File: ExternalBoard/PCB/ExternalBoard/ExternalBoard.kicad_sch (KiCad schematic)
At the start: 2 parts, among them U1 REF01CP

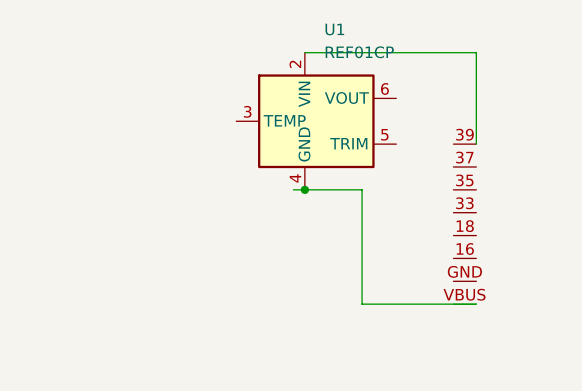
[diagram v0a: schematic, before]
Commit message: 5
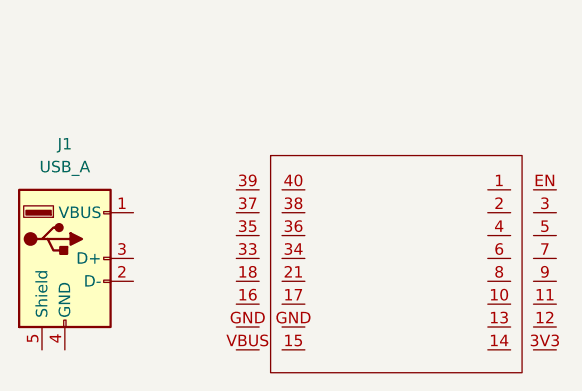
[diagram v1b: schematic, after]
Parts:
- removed U1: REF01CP, Package_DIP:DIP-8_W7.62mm, symbol Reference_Voltage:REF01CP
- added J1: USB_A, Connector_USB:USB_A_Connfly_DS1095, symbol Connector:USB_A
- D1: footprint ESP32_S2:ESP32_S2 -> (none)
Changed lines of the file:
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@@
 	(generator_version "9.0")
 	(paper "A4")
-	(junction
-		(at 96.52 99.06)
-		(diameter 0)
-		(color 0 0 0 0)
-	)
-	(wire
-		(pts
-			(xy 95.25 99.06) (xy 96.52 99.06)
+	(symbol
+		(lib_id "Connector:USB_A")
+		(at 69.85 106.68 0)
+		(unit 1)
+		(exclude_from_sim no)
+		(in_bom yes)
+		(on_board yes)
+		(dnp no)
+		(fields_autoplaced yes)
+		(property "Reference" "J1"
+			(at 69.85 93.98 0)
+			(effects
+				(font
+					(size 1.27 1.27)
+				)
+			)
 		)
-		(stroke
-			(width 0)
-			(type default)
+		(property "Value" "USB_A"
+			(at 69.85 96.52 0)
+			(effects
+				(font
+					(size 1.27 1.27)
+				)
+			)
 		)
-	)
-	(wire
-		(pts
-			(xy 102.87 99.06) (xy 102.87 111.76)
+		(property "Footprint" "Connector_USB:USB_A_Connfly_DS1095"
+			(at 73.66 107.95 0)
+			(effects
+				(font
+					(size 1.27 1.27)
+				)
+				(hide yes)
+			)
 		)
-		(stroke
-			(width 0)
-			(type default)
+		(property "Datasheet" "~"
+			(at 73.66 107.95 0)
+			(effects
+				(font
+					(size 1.27 1.27)
+				)
+				(hide yes)
+			)
 		)
-	)
-	(wire
-		(pts
-			(xy 102.87 111.76) (xy 115.57 111.76)
+		(property "Description" "USB Type A connector"
+			(at 69.85 106.68 0)
+			(effects
+				(font
+					(size 1.27 1.27)
+				)
+				(hide yes)
+			)
 		)
-		(stroke
-			(width 0)
-			(type default)
+		(pin "2"
 		)
-	)
-	(wire
-		(pts
-			(xy 96.52 99.06) (xy 102.87 99.06)
+		(pin "3"
 		)
-		(stroke
-			(width 0)
-			(type default)
+		(pin "5"
 		)
-	)
-	(wire
-		(pts
-			(xy 115.57 83.82) (xy 115.57 93.98)
+		(pin "1"
 		)
-		(stroke
-			(width 0)
-			(type default)
+		(pin "4"
 		)
-	)
-	(wire
-		(pts
-			(xy 96.52 83.82) (xy 115.57 83.82)
-		)
-		(stroke
-			(width 0)
-			(type default)
+		(instances
+			(project ""
+				(path "/1428142b-2c57-4b00-8cf4-1baa0f3d7ee6"
+					(reference "J1")
+					(unit 1)
+				)
+			)
 		)
 	)
 	(symbol
 		(lib_id "ESP32_S2:ESP32_S2")
-		(at 135.89 102.87 0)
+		(at 106.68 106.68 0)
 		(unit 1)
 		(exclude_from_sim no)
@@
 		(fields_autoplaced yes)
 		(property "Reference" "D1"
-			(at 135.89 102.87 0)
+			(at 107.95 107.95 0)
 			(effects
 				(font
@@
 		)
 		(property "Value" "~"
-			(at 113.03 91.44 0)
+			(at 106.68 92.71 0)
 			(effects
 				(font
@@
 			)
 		)
-		(property "Footprint" "ESP32_S2:ESP32_S2"
-			(at 135.89 102.87 0)
+		(property "Footprint" ""
+			(at 106.68 106.68 0)
 			(effects
 				(font
@@
 		)
 		(property "Datasheet" ""
-			(at 135.89 102.87 0)
+			(at 106.68 106.68 0)
 			(effects
 				(font
@@
 		)
 		(property "Description" ""
-			(at 135.89 102.87 0)
+			(at 106.68 106.68 0)
 			(effects
 				(font
@@
 			)
 		)
-		(pin "39"
+		(pin "21"
+		)
+		(pin "GND"
 		)
 		(pin "VBUS"
 		)
-		(pin "16"
+		(pin "4"
 		)
 		(pin "37"
 		)
-		(pin "35"
+		(pin "2"
+		)
+		(pin "39"
+		)
+		(pin "33"
+		)
+		(pin "16"
 		)
 		(pin "GND"
 		)
+		(pin "40"
+		)
 		(pin "18"
 		)
-		(pin "33"
+		(pin "38"
+		)
+		(pin "36"
+		)
+		(pin "34"
+		)
+		(pin "35"
+		)
+		(pin "17"
+		)
+		(pin "15"
+		)
+		(pin "1"
+		)
+		(pin "10"
+		)
+		(pin "9"
+		)
+		(pin "7"
+		)
+		(pin "11"
+		)
+		(pin "EN"
+		)
+		(pin "3"
+		)
+		(pin "14"
+		)
+		(pin "3V3"
+		)
+		(pin "13"
+		)
+		(pin "6"
+		)
+		(pin "12"
+		)
+		(pin "8"
+		)
+		(pin "5"
 		)
 		(instances
@@
 					(unit 1)
 				)
-			)
-		)
-	)
-	(symbol
-		(lib_id "Reference_Voltage:REF01CP")
-		(at 96.52 91.44 0)
-		(unit 1)
-		(exclude_from_sim no)
-		(in_bom yes)
-		(on_board yes)
-		(dnp no)
-		(fields_autoplaced yes)
-		(property "Reference" "U1"
-			(at 98.6633 81.28 0)
-			(effects
-				(font
-					(size 1.27 1.27)
-				)
-				(justify left)
-			)
-		)
-		(property "Value" "REF01CP"
-			(at 98.6633 83.82 0)
-			(effects
-				(font
-					(size 1.27 1.27)
-				)
-				(justify left)
-			)
-		)
-		(property "Footprint" "Package_DIP:DIP-8_W7.62mm"
-			(at 111.76 97.79 0)
-			(effects
-				(font
-					(size 1.27 1.27)
-					(italic yes)
-				)
-				(hide yes)
-			)
-		)
-		(property "Datasheet" "https://www.analog.com/media/en/technical-documentation/data-sheets/REF01_02_03.pdf"
-			(at 97.79 91.44 0)
-			(effects
-				(font
-					(size 1.27 1.27)
-					(italic yes)
-				)
-				(hide yes)
-			)
-		)
-		(property "Description" "10V ±100mV Precision Voltage Reference, PDIP-8"
-			(at 96.52 91.44 0)
-			(effects
-				(font
-					(size 1.27 1.27)
-				)
-				(hide yes)
-			)
-		)
-		(pin "5"
-		)
-		(pin "6"
-		)
-		(pin "4"
-		)
-		(pin "8"
-		)
-		(pin "3"
-		)
-		(pin "2"
-		)
-		(pin "7"
-		)
-		(pin "1"
-		)
-		(instances
-			(project ""
-				(path "/1428142b-2c57-4b00-8cf4-1baa0f3d7ee6"
-					(reference "U1")
-					(unit 1)
-				)

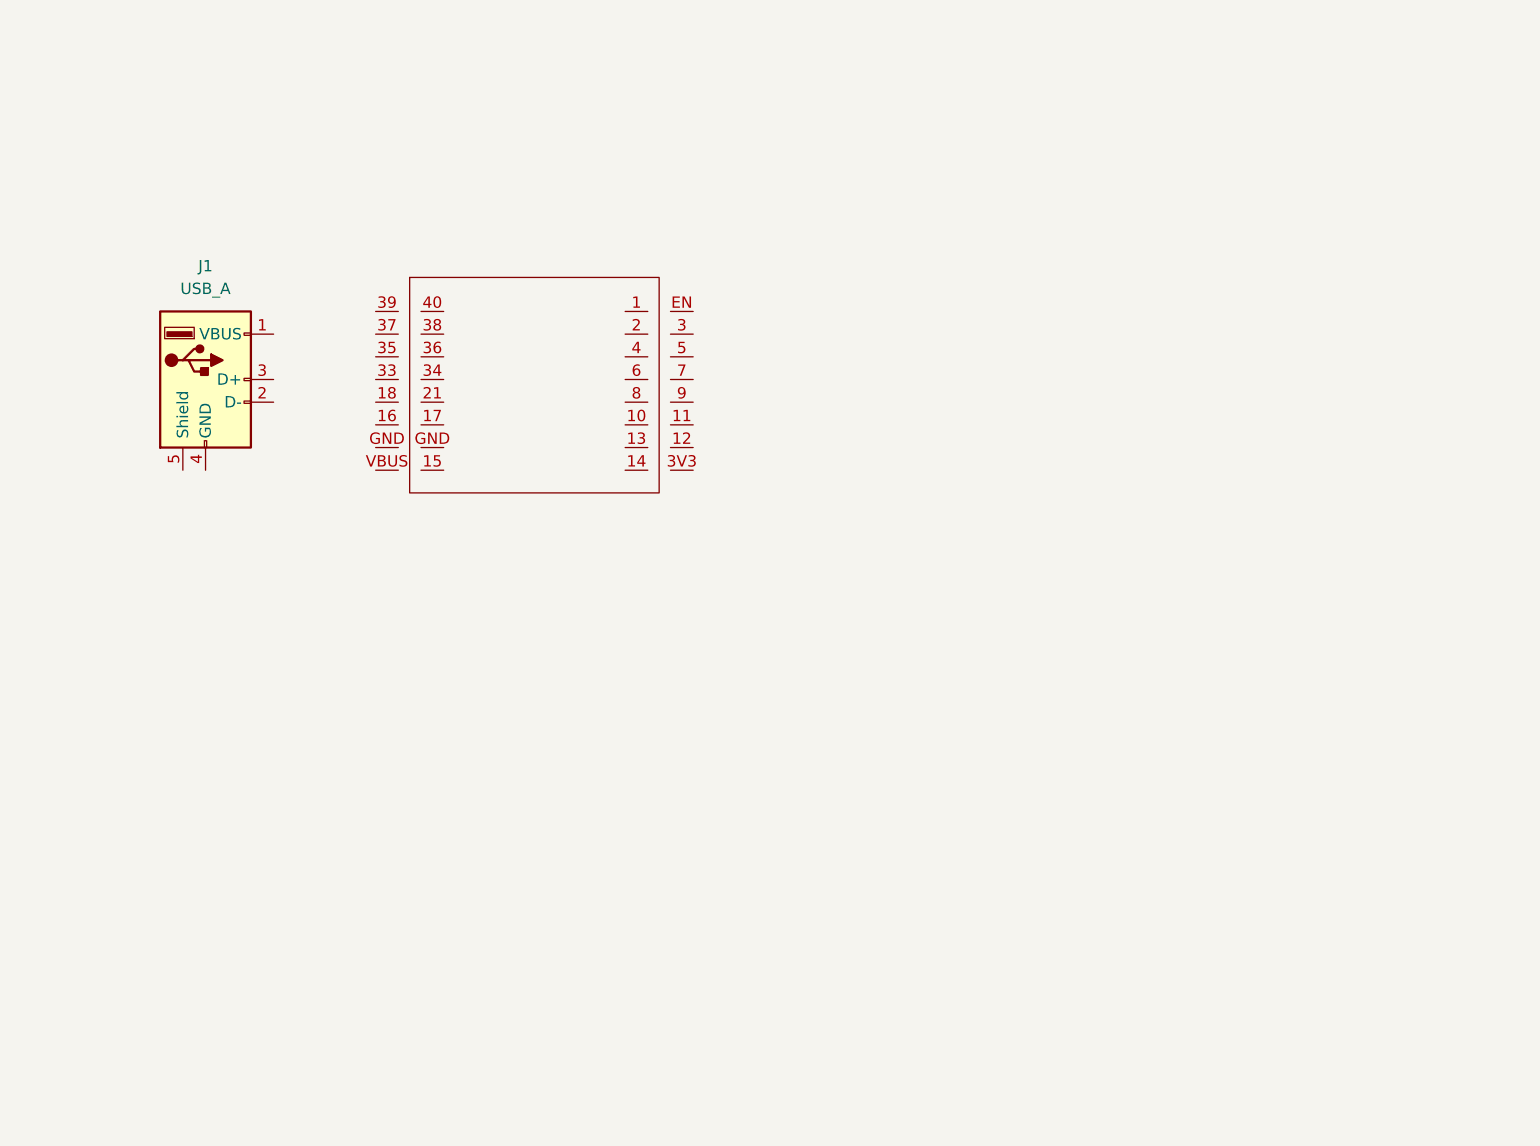
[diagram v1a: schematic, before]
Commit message: 3
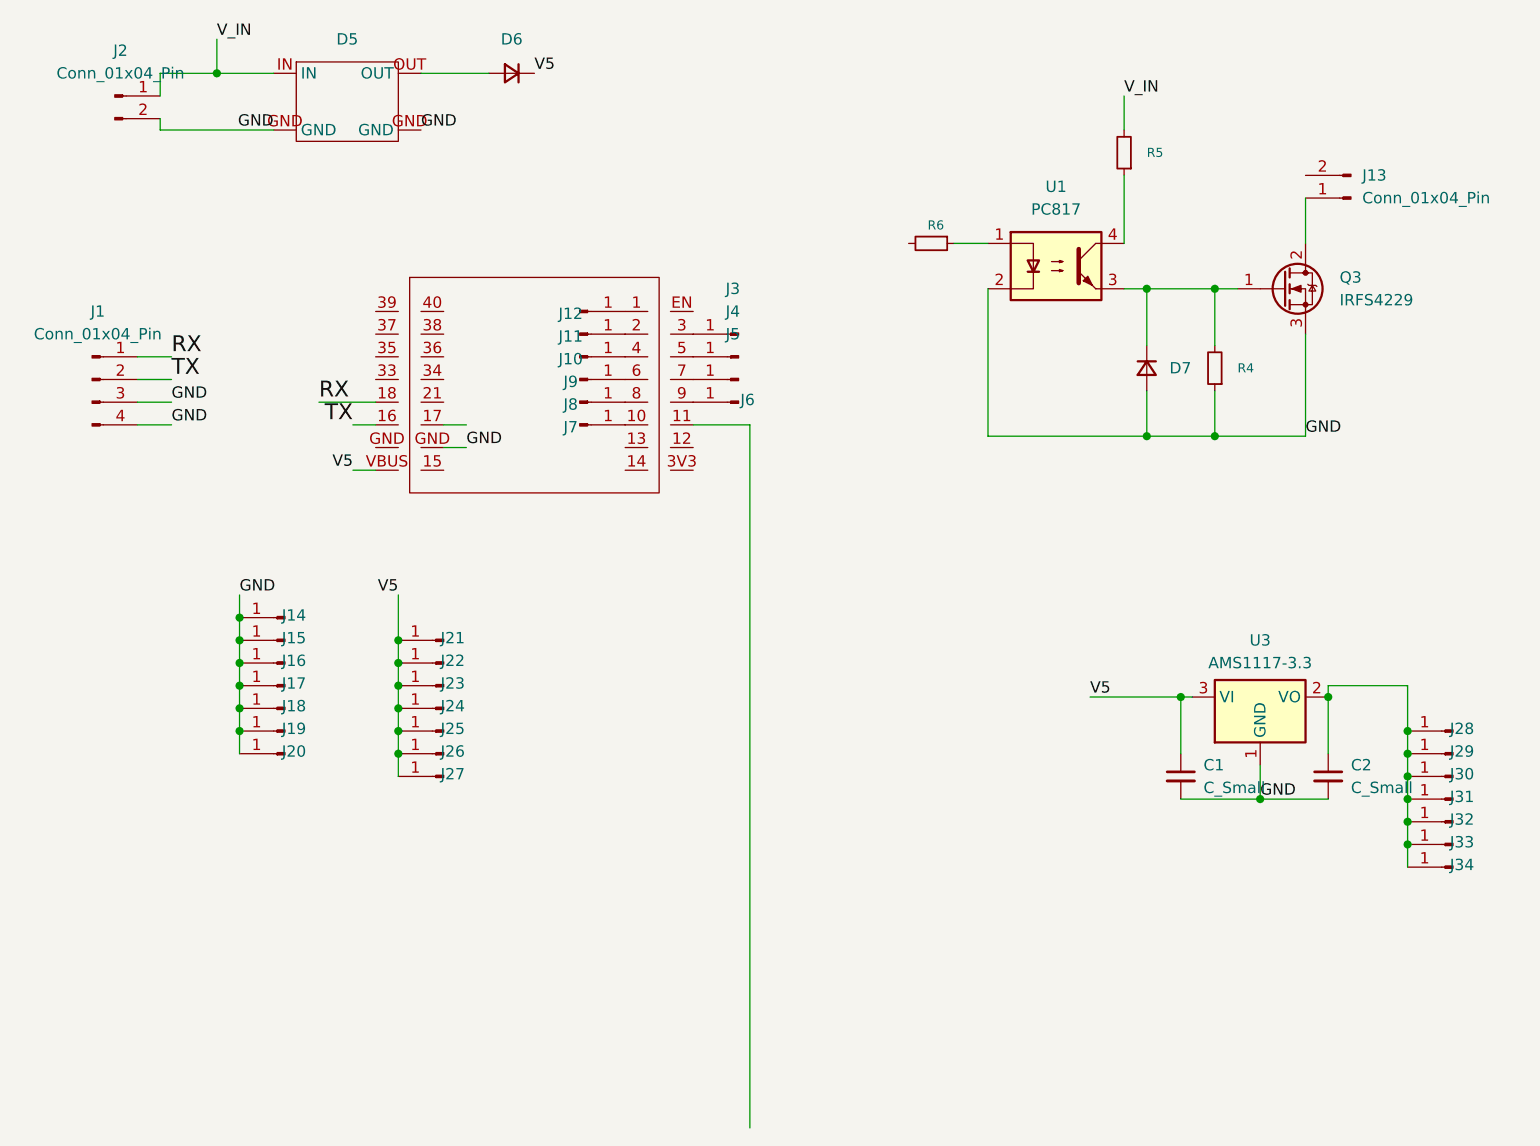
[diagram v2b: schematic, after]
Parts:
- removed J1: USB_A, Connector_USB:USB_A_Connfly_DS1095, symbol Connector:USB_A
- added C1, C2: C_Small, Capacitor_SMD:C_1206_3216Metric, symbol Device:C_Small
- added D5: (no value), ESP32_S2:StepDown, symbol ESP32_S2:StepDown
- added D6: D_Small, Diode_SMD:D_SMA, symbol Device:D_Small
- added D7: D_Small, Diode_SMD:D_SMF, symbol Device:D_Small
- added J1: Conn_01x04_Pin, Connector_PinHeader_2.54mm:PinHeader_1x04_P2.54mm_Vertical, symbol Connector:Conn_01x04_Pin
- added J10, J11, J12, J14, J15, J16, J17, J18, J19, J20, J21, J22, J23, J24, J25, J26, J27, J28, J29, J3, J30, J31, J32, J33, J34, J4, J5, J6, J7, J8, J9: Conn_01x04_Pin, ESP32_S2:PIN0, symbol Connector:Conn_01x01_Pin
- added J13, J2: Conn_01x04_Pin, Connector_PinHeader_2.54mm:PinHeader_1x02_P2.54mm_Vertical, symbol Connector:Conn_01x02_Pin
- added Q3: IRFS4229, Package_TO_SOT_SMD:TO-263-2, symbol Transistor_FET:IRFS4229
- added R4, R5, R6: R_Small, Resistor_SMD:R_1206_3216Metric_Pad1.30x1.75mm_HandSolder, symbol Device:R_Small
- added U1: PC817, Package_DIP:DIP-4_W7.62mm, symbol Isolator:PC817
- added U3: AMS1117-3.3, Package_TO_SOT_SMD:SOT-223-3_TabPin2, symbol Regulator_Linear:AMS1117-3.3
- D1: value ~ -> (none); footprint (none) -> ESP32_S2:ESP32_S2_V2
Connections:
- net at D1.1: now also J12.1 (Pin_1)
- net at D1.10: now also J7.1 (Pin_1)
- net TX: now reaches D1.16
- net TX: now also J1.2 (Pin_2)
- net RX: now reaches D1.18
- net RX: now also J1.1 (Pin_1)
- net at D1.2: now also J11.1 (Pin_1)
- net at D1.3: now also J3.1 (Pin_1)
- net at D1.4: now also J10.1 (Pin_1)
- net at D1.5: now also J4.1 (Pin_1)
- net at D1.6: now also J9.1 (Pin_1)
- net at D1.7: now also J5.1 (Pin_1)
- net at D1.8: now also J8.1 (Pin_1)
- net at D1.9: now also J6.1 (Pin_1)
- net GND: now reaches D1.GND
- net GND: now also C1.2, C2.2, D5.GND, D7.2 (A), J1.3 (Pin_3), J1.4 (Pin_4), J14.1 (Pin_1), J15.1 (Pin_1), J16.1 (Pin_1), J17.1 (Pin_1), J18.1 (Pin_1), J19.1 (Pin_1), J2.2 (Pin_2), J20.1 (Pin_1), Q3.3 (S), R4.1, U1.2, U3.1 (GND)
- net V5: now reaches D1.VBUS
- net V5: now also C1.1, D6.1 (K), J21.1 (Pin_1), J22.1 (Pin_1), J23.1 (Pin_1), J24.1 (Pin_1), J25.1 (Pin_1), J26.1 (Pin_1), J27.1 (Pin_1), U3.3 (VI)
- new net: C2.1, J28.1 (Pin_1), J29.1 (Pin_1), J30.1 (Pin_1), J31.1 (Pin_1), J32.1 (Pin_1), J33.1 (Pin_1), J34.1 (Pin_1), U3.2 (VO)
- new net: R6.1, U1.1
- new net: D7.1 (K), Q3.1 (G), R4.2, U1.3
- new net: R5.1, U1.4
- new net: D5.OUT, D6.2 (A)
- new net: J13.1 (Pin_1), Q3.2 (D)
- new net V_IN: D5.IN, J2.1 (Pin_1), R5.2
